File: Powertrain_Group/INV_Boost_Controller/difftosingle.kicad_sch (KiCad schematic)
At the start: 10 parts, among them U1 INA333AIDGK

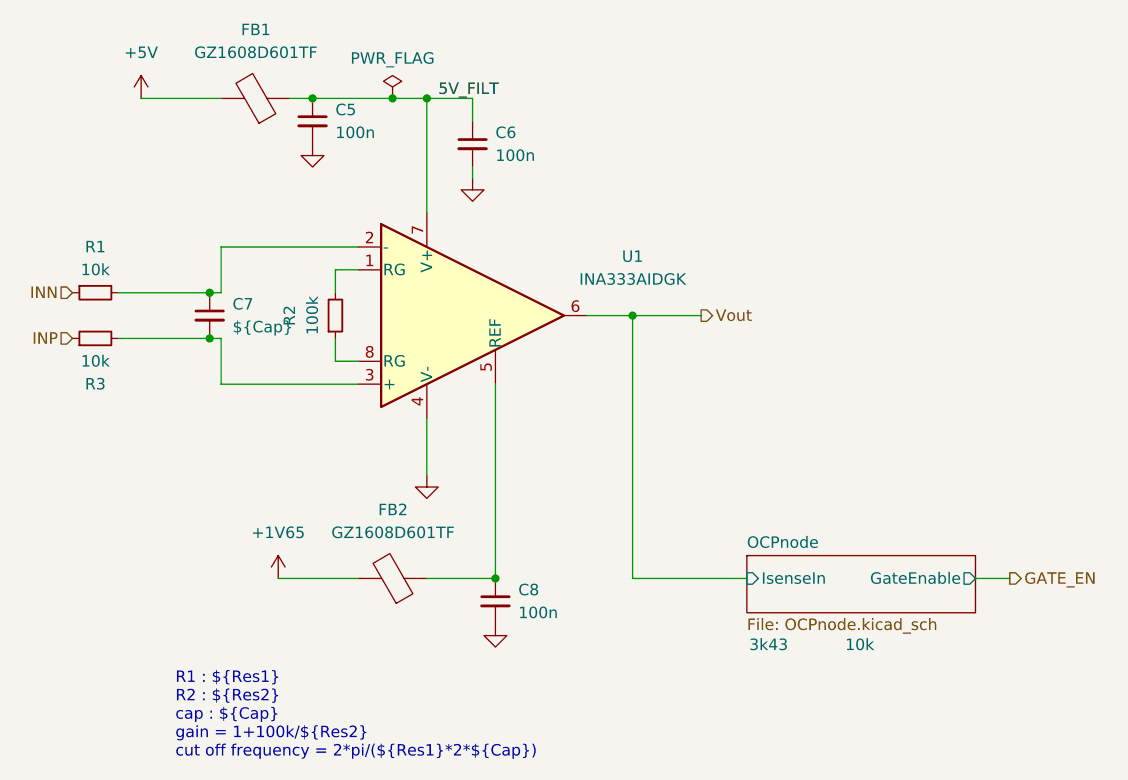
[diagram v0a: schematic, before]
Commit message: [INV_Boost_Controller] V1.1
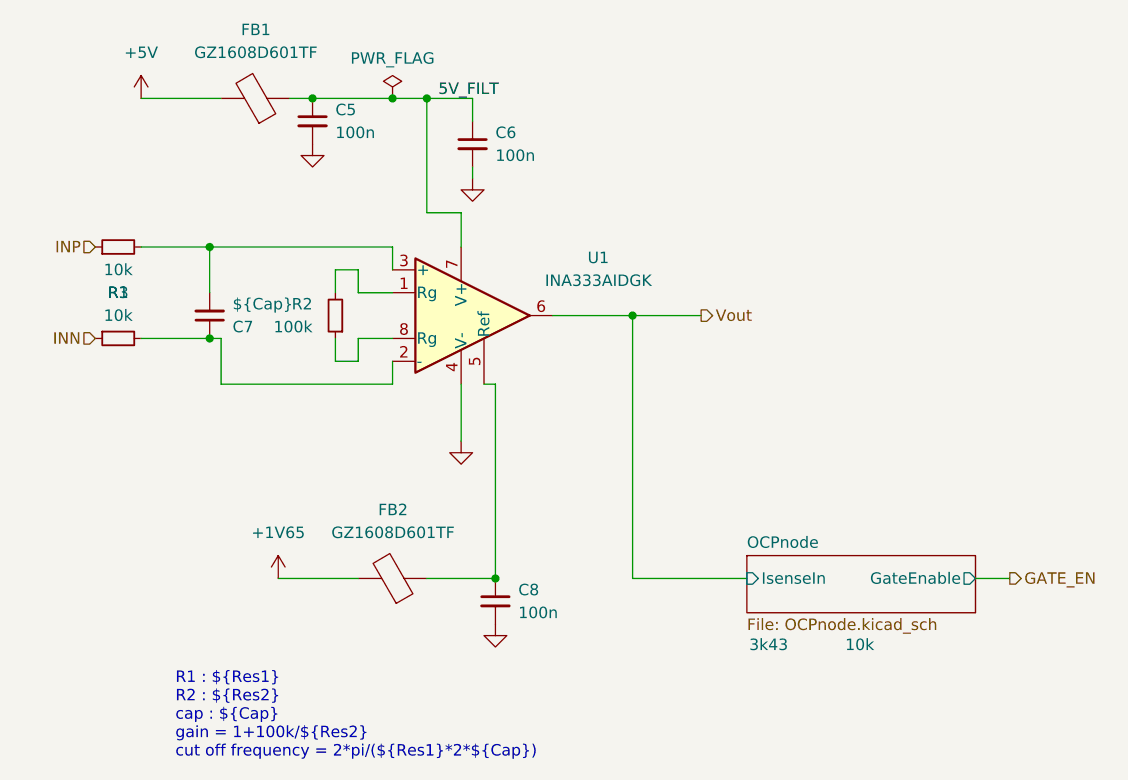
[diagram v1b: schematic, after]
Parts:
- U1: footprint PCM_Package_SO_AKL:MSOP-8_3x3mm_P0.65mm -> Package_SO:VSSOP-8_3x3mm_P0.65mm; symbol PCM_Amplifier_Instrumentation_AKL:INA333AIDGK -> Amplifier_Instrumentation:INA333xxDGK
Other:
- company: (none) -> NTURacing
- title: (none) -> INV_Boost_Controller
- moved on the sheet: R1, R2, R3

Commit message: [INV_Boost_Controller] V1.1 again
minor update for jlc
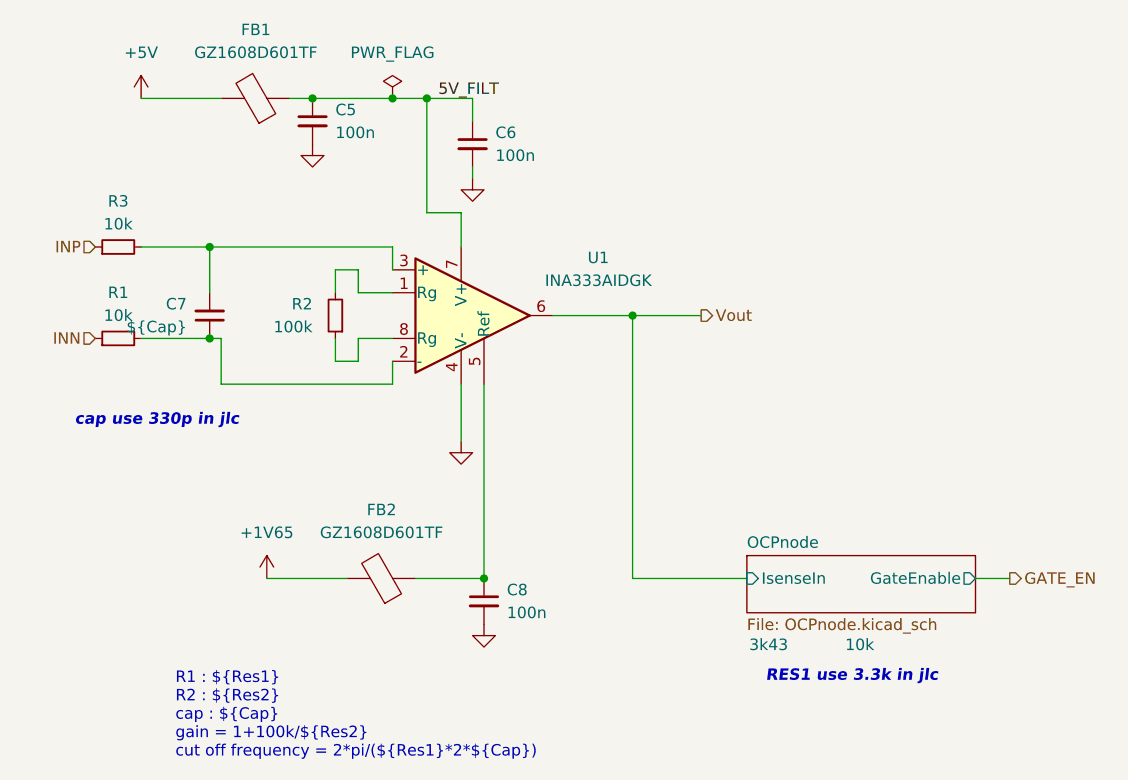
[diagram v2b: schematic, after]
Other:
- note added: "RES1 use 3.3k in jlc"
- note added: "cap use 330p in jlc"
- moved on the sheet: C8, FB2
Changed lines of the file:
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@@
+		)
+	)
+	(text "cap use 330p in jlc "
+		(exclude_from_sim no)
+		(at 88.138 91.694 0)
+		(effects
+			(font
+				(size 1.27 1.27)
+				(thickness 0.254)
+				(bold yes)
+				(italic yes)
+			)
+		)
+	)
+	(text "RES1 use 3.3k in jlc "
+		(exclude_from_sim no)
+		(at 165.354 120.142 0)
+		(effects
+			(font
+				(size 1.27 1.27)
+				(thickness 0.254)
+				(bold yes)
+				(italic yes)
+			)
 		)
 	)
 	(junction
-		(at 125.73 109.22)
+		(at 124.46 109.22)
 		(diameter 0)
 		(color 0 0 0 0)
@@
 	(wire
 		(pts
-			(xy 101.6 109.22) (xy 110.49 109.22)
+			(xy 100.33 109.22) (xy 109.22 109.22)
 		)
 		(stroke
@@
 	(wire
 		(pts
-			(xy 118.11 109.22) (xy 125.73 109.22)
+			(xy 116.84 109.22) (xy 124.46 109.22)
 		)
 		(stroke
@@
 	(wire
 		(pts
-			(xy 125.73 87.63) (xy 125.73 109.22)
+			(xy 124.46 87.63) (xy 124.46 109.22)
 		)
 		(stroke
@@
 		(pts
 			(xy 123.19 58.42) (xy 123.19 55.88)
-		)
-		(stroke
-			(width 0)
-			(type default)
-		)
-	)
-	(wire
-		(pts
-			(xy 124.46 87.63) (xy 125.73 87.63)
 		)
 		(stroke
@@
 		(on_board yes)
 		(dnp no)
+		(fields_autoplaced yes)
 		(property "Reference" "C5"
-			(at 107.95 57.1563 0)
+			(at 107.95 57.1562 0)
 			(effects
 				(font
@@
 		)
 		(property "Value" "100n"
-			(at 107.95 59.6963 0)
+			(at 107.95 59.6962 0)
 			(effects
 				(font
@@
 	(symbol
 		(lib_id "power:GND")
-		(at 125.73 114.3 0)
+		(at 124.46 114.3 0)
 		(unit 1)
 		(exclude_from_sim no)
@@
 		(fields_autoplaced yes)
 		(property "Reference" "#PWR029"
-			(at 125.73 120.65 0)
+			(at 124.46 120.65 0)
 			(effects
 				(font
@@
 		)
 		(property "Value" "GND"
-			(at 125.73 119.38 0)
+			(at 124.46 119.38 0)
 			(effects
 				(font
@@
 		)
 		(property "Footprint" ""
-			(at 125.73 114.3 0)
+			(at 124.46 114.3 0)
 			(effects
 				(font
@@
 		)
 		(property "Datasheet" ""
-			(at 125.73 114.3 0)
+			(at 124.46 114.3 0)
 			(effects
 				(font
@@
 		)
 		(property "Description" "Power symbol creates a global label with name \"GND\" , ground"
-			(at 125.73 114.3 0)
+			(at 124.46 114.3 0)
 			(effects
 				(font
@@
 	(symbol
 		(lib_id "Device:FerriteBead")
-		(at 114.3 109.22 270)
+		(at 113.03 109.22 270)
 		(mirror x)
 		(unit 1)
@@
 		(on_board yes)
 		(dnp no)
+		(fields_autoplaced yes)
 		(property "Reference" "FB2"
-			(at 114.3508 101.6 90)
+			(at 113.0808 101.6 90)
 			(effects
 				(font
@@
 		)
 		(property "Value" "GZ1608D601TF"
-			(at 114.3508 104.14 90)
+			(at 113.0808 104.14 90)
 			(effects
 				(font
@@
 		)
 		(property "Footprint" "Capacitor_SMD:C_0603_1608Metric"
-			(at 114.3 110.998 90)
+			(at 113.03 110.998 90)
 			(effects
 				(font
@@
 		)
 		(property "Datasheet" "~"
-			(at 114.3 109.22 0)
+			(at 113.03 109.22 0)
 			(effects
 				(font
@@
 		)
 		(property "Description" "Ferrite bead"
-			(at 114.3 109.22 0)
+			(at 113.03 109.22 0)
 			(effects
 				(font
@@
 		(on_board yes)
 		(dnp no)
+		(fields_autoplaced yes)
 		(property "Reference" "FB1"
 			(at 99.1108 48.26 90)
@@
 		(on_board yes)
 		(dnp no)
+		(fields_autoplaced yes)
 		(property "Reference" "#FLG01"
 			(at 114.3 53.975 0)
@@
 		)
 		(property "Value" "PWR_FLAG"
-			(at 114.3 51.435 0)
+			(at 114.3 50.8 0)
 			(effects
 				(font
@@
 	(symbol
 		(lib_id "power:+1V35")
-		(at 101.6 109.22 0)
+		(at 100.33 109.22 0)
 		(unit 1)
 		(exclude_from_sim no)
@@
 		(fields_autoplaced yes)
 		(property "Reference" "#PWR028"
-			(at 101.6 113.03 0)
+			(at 100.33 113.03 0)
 			(effects
 				(font
@@
 		)
 		(property "Value" "+1V65"
-			(at 101.6 104.14 0)
+			(at 100.33 104.14 0)
 			(effects
 				(font
@@
 		)
 		(property "Footprint" ""
-			(at 101.6 109.22 0)
+			(at 100.33 109.22 0)
 			(effects
 				(font
@@
 		)
 		(property "Datasheet" ""
-			(at 101.6 109.22 0)
+			(at 100.33 109.22 0)
 			(effects
 				(font
@@
 		)
 		(property "Description" "Power symbol creates a global label with name \"+1V35\""
-			(at 101.6 109.22 0)
+			(at 100.33 109.22 0)
 			(effects
 				(font
@@
 		(on_board yes)
 		(dnp no)
+		(fields_autoplaced yes)
 		(property "Reference" "C7"
-			(at 96.52 81.2737 0)
-			(effects
-				(font
-					(size 1.27 1.27)
-				)
-				(justify left)
+			(at 91.44 78.7335 0)
+			(effects
+				(font
+					(size 1.27 1.27)
+				)
+				(justify right)
 			)
 		)
 		(property "Value" "${Cap}"
-			(at 96.52 78.7337 0)
-			(effects
-				(font
-					(size 1.27 1.27)
-				)
-				(justify left)
+			(at 91.44 81.2735 0)
+			(effects
+				(font
+					(size 1.27 1.27)
+				)
+				(justify right)
 			)
 		)
@@
 		(lib_id "Device:R_Small")
 		(at 83.82 82.55 90)
-		(mirror x)
 		(unit 1)
 		(exclude_from_sim no)
@@
 		(on_board yes)
 		(dnp no)
+		(fields_autoplaced yes)
 		(property "Reference" "R1"
 			(at 83.82 77.47 90)
@@
 		(on_board yes)
 		(dnp no)
+		(fields_autoplaced yes)
 		(property "Reference" "R3"
-			(at 83.82 77.47 90)
+			(at 83.82 67.31 90)
 			(effects
 				(font
@@
 		)
 		(property "Value" "10k"
-			(at 83.82 74.93 90)
+			(at 83.82 69.85 90)
 			(effects
 				(font
@@
 		(fields_autoplaced yes)
 		(property "Reference" "C6"
-			(at 125.73 59.6963 0)
+			(at 125.73 59.6962 0)
 			(effects
 				(font
@@
 		)
 		(property "Value" "100n"
-			(at 125.73 62.2363 0)
+			(at 125.73 62.2362 0)
 			(effects
 				(font
@@
 	(symbol
 		(lib_id "Device:C_Small")
-		(at 125.73 111.76 0)
+		(at 124.46 111.76 0)
 		(unit 1)
 		(exclude_from_sim no)
@@
 		(on_board yes)
 		(dnp no)
+		(fields_autoplaced yes)
 		(property "Reference" "C8"
-			(at 128.27 110.4963 0)
+			(at 127 110.4962 0)
 			(effects
 				(font
@@
 		)
 		(property "Value" "100n"
-			(at 128.27 113.0363 0)
+			(at 127 113.0362 0)
 			(effects
 				(font
@@
 		)
 		(property "Footprint" "Capacitor_SMD:C_0402_1005Metric"
-			(at 125.73 111.76 0)
+			(at 124.46 111.76 0)
 			(effects
 				(font
@@
 		)
 		(property "Datasheet" "~"
-			(at 125.73 111.76 0)
+			(at 124.46 111.76 0)
 			(effects
 				(font
@@
 		)
 		(property "Description" "Unpolarized capacitor, small symbol"
-			(at 125.73 111.76 0)
+			(at 124.46 111.76 0)
 			(effects
 				(font
@@
 		(on_board yes)
 		(dnp no)
+		(fields_autoplaced yes)
 		(stroke
 			(width 0.1524)
